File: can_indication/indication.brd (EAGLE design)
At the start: 63.5 x 38 mm, 51 parts, among them CON1 SM04B-GHS-TB, CON2 SM04B-GHS-TB, U1 STM32F103CB

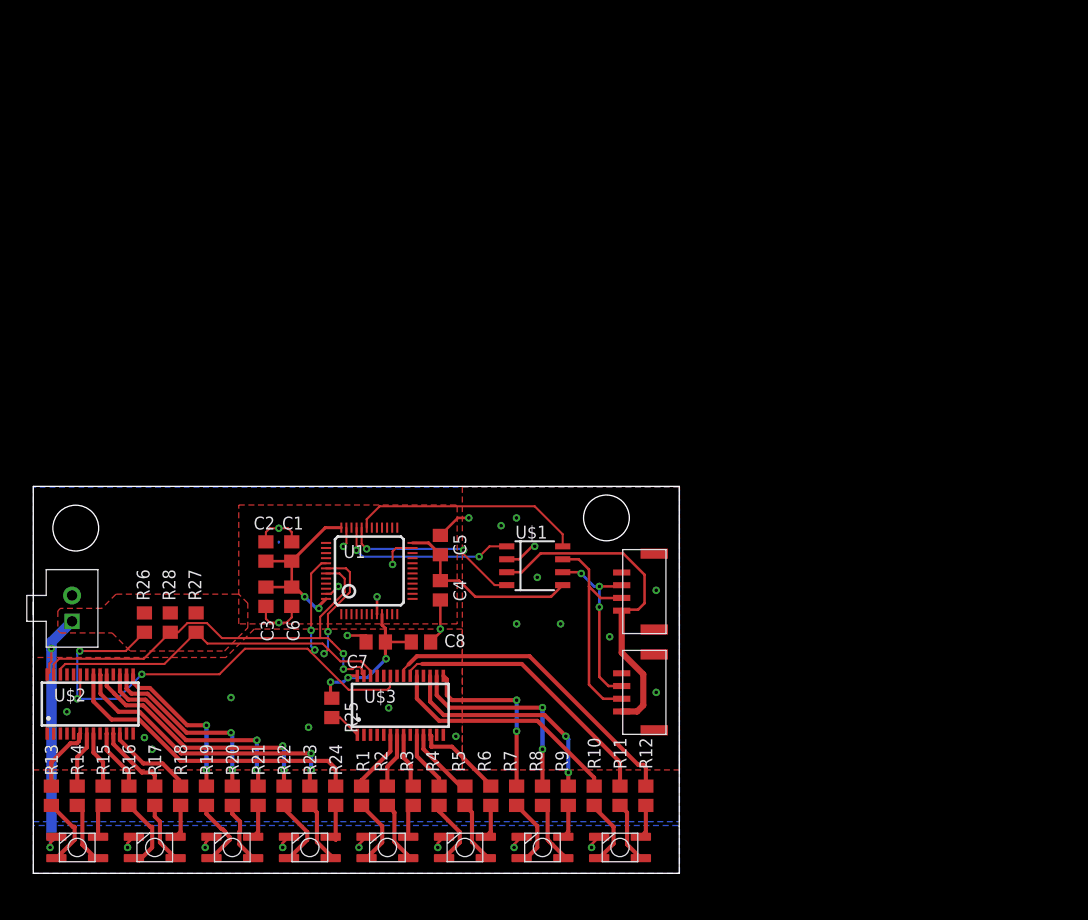
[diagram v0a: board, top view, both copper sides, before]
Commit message: Changed the indication board so it uses higher power LED's now
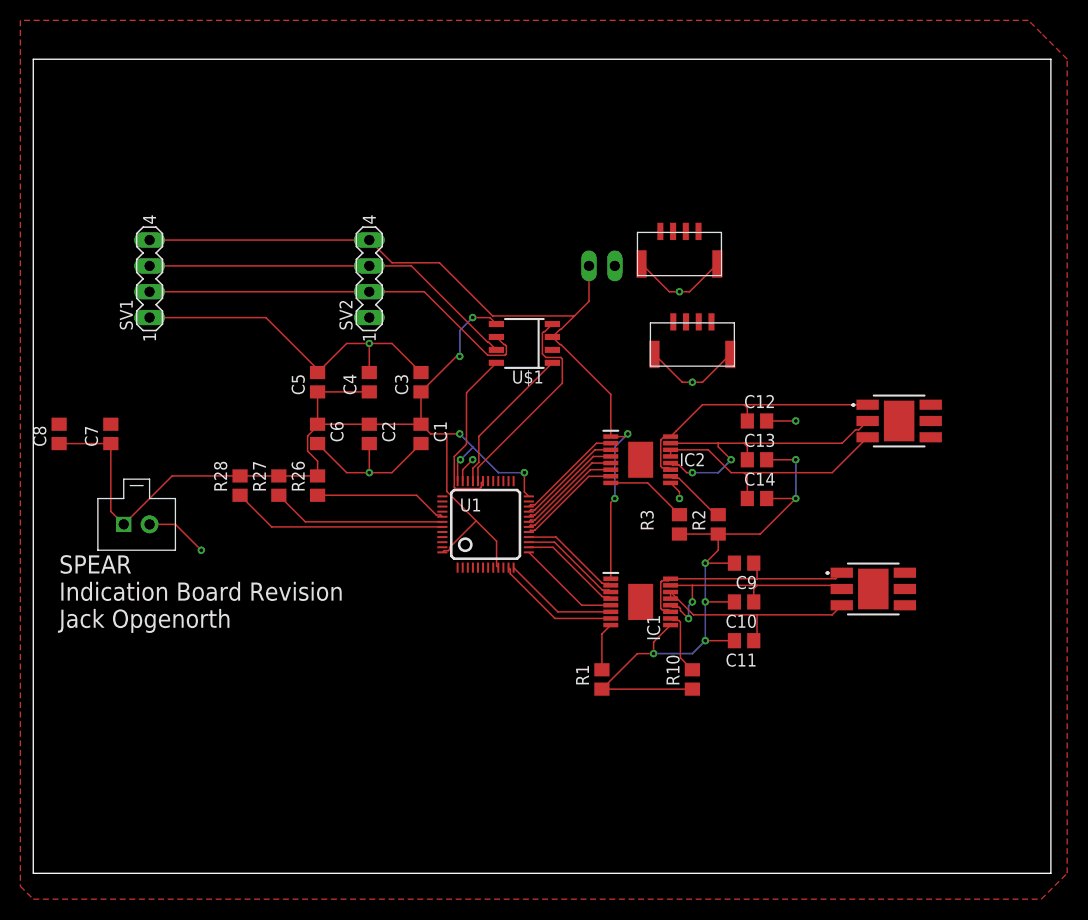
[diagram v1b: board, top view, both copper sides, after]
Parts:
- removed D1, D2, D3, D4, D5, D6, D7, D8: CLV1L-FKB-CHMMQEHBB7673673, SPEAR:PLCC-4
- removed R11, R12, R14, R15, R17, R18, R20, R21, R23, R24, R5, R6, R8, R9: 10, resistor:R0805
- removed R13, R16, R19, R22, R4, R7: 66, resistor:R0805
- removed R25: 10K, resistor:R0805
- removed U$2, U$3: PCA9685PW, SPEAR:TSSOP28
- added C10, C11, C12, C13, C14, C9: (no value), rcl:C0805
- added IC1, IC2: TPS92630QPWPRQ1, TPS92630QPWPRQ1:SOP65P640X120-17N
- added JP1: (no value), pinhead:1X02
- added LED1, LED2: AAAF5051-05, AAAF5051-05:AAAF505105
- added SV1, SV2: (no value), con-lstb:MA04-1
- R1: value 66 -> 10K
- R10: value 66 -> 815
- R2: value 10 -> 815
- R3: value 10 -> 10K
- moved R2 42.1 mm to (67.3, 34.3), turned to 90 degrees
- moved C8 41.0 mm to (2.54, 43.2), turned to 90 degrees
- moved R3 37.4 mm to (63.5, 34.3), turned to 90 degrees
- moved CON1 36.1 mm to (64.8, 53.3), turned to 0 degrees
- moved CON2 34.9 mm to (63.5, 62.2), turned to 0 degrees
- moved C7 33.1 mm to (7.62, 43.2), turned to 90 degrees
- moved R1 26.2 mm to (55.9, 19.1), turned to 90 degrees
- moved C3 26.0 mm to (38.1, 48.3), turned to 90 degrees
- moved U$1 21.9 mm to (48.3, 52.1), turned to 90 degrees
- moved R26 21.7 mm to (27.9, 38.1)
- moved C4 21.6 mm to (33.0, 48.3), turned to 90 degrees
- moved C5 20.0 mm to (27.9, 48.3)
- moved C1 17.2 mm to (38.1, 43.2), turned to 270 degrees
- moved C6 16.2 mm to (27.9, 43.2)
- moved R27 15.7 mm to (24.1, 38.1)
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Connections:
- removed net LEDA0: R13.1, U$2.6
- removed net LEDA1: R14.1, U$2.7
- removed net LEDA10: R21.1, U$2.17
- removed net LEDA11: U$2.18
- removed net LEDA12: R22.1, U$2.19
- removed net LEDA13: R23.1, U$2.20
- removed net LEDA14: R24.1, U$2.21
- removed net LEDA15: U$2.22
- removed net LEDA2: R15.1, U$2.8
- removed net LEDA3: U$2.9
- removed net LEDA4: R16.1, U$2.10
- removed net LEDA5: R17.1, U$2.11
- removed net LEDA6: R18.1, U$2.12
- removed net LEDA7: U$2.13
- removed net LEDA8: R19.1, U$2.15
- removed net LEDA9: R20.1, U$2.16
- removed net LEDB0: R1.1, U$3.6
- removed net LEDB1: R2.1, U$3.7
- removed net LEDB10: R9.1, U$3.17
- removed net LEDB11: U$3.18
- removed net LEDB12: R10.1, U$3.19
- removed net LEDB13: R11.1, U$3.20
- removed net LEDB14: R12.1, U$3.21
- removed net LEDB15: U$3.22
- removed net LEDB2: R3.1, U$3.8
- removed net LEDB3: U$3.9
- removed net LEDB4: R4.1, U$3.10
- removed net LEDB5: R5.1, U$3.11
- removed net LEDB6: R6.1, U$3.12
- removed net LEDB7: U$3.13
- removed net LEDB8: R7.1, U$3.15
- removed net LEDB9: R8.1, U$3.16
- removed net N$10: D8.P$2, R10.2
- removed net N$11: D8.P$3, R11.2
- removed net N$13: D1.P$2, R13.2
- removed net N$15: D1.P$4, R15.2
- removed net N$16: D2.P$2, R16.2
- removed net N$17: D2.P$3, R17.2
- removed net N$18: D2.P$4, R18.2
- removed net N$19: D3.P$2, R19.2
- removed net N$20: D3.P$3, R20.2
- removed net N$21: D3.P$4, R21.2
- removed net N$22: D4.P$2, R22.2
- removed net N$23: D4.P$3, R23.2
- removed net N$24: D4.P$4, R24.2
- removed net N$27: R25.2, U$3.1
- removed net N$4: D6.P$2, R4.2
- removed net N$5: D6.P$3, R5.2
- removed net N$6: D6.P$4, R6.2
- removed net N$7: D7.P$2, R7.2
- removed net N$8: D7.P$3, R8.2
- removed net N$9: D7.P$4, R9.2
- new net L1OUT1: C9.1, IC1.11, IC1.16, LED1.1
- new net L1OUT2: C10.1, IC1.12, IC1.15, LED1.2
- new net L1OUT3: C11.1, IC1.13, IC1.14, LED1.3
- new net L2OUT1: C12.1, IC2.11, IC2.16, LED2.1
- new net L2OUT2: C13.1, IC2.12, IC2.15, LED2.2
- new net L2OUT3: C14.1, IC2.13, IC2.14, LED2.3
- new net PA1: IC1.7, U1.11
- new net PA2: IC1.6, U1.12
- new net PA3: IC1.5, U1.13
- new net PA4: IC1.4, U1.14
- new net PA5: IC1.3, U1.15
- new net PA6: IC1.2, U1.16
- new net PA7: IC2.7, U1.17
- new net PB0: IC2.6, U1.18
- new net PB1: IC2.5, U1.19
- new net PB10: IC2.3, U1.21
- new net PB11: IC2.2, U1.22
- new net PB2: IC2.4, U1.20
- new net PB8: U1.45
- net +3V3: no longer D1.P$1, D2.P$1, D3.P$1, D4.P$1, D5.P$1, D6.P$1, D7.P$1, D8.P$1, R25.1, U$2.28, U$3.28
- net +5V: now also IC1.1, IC2.1, JP1.1, SV1.4, SV2.4; no longer CON1.P$1, CON2.P$1
- net CANH: now also SV1.3, SV2.3; no longer CON1.P$2, CON2.P$2
- net CANL: now also SV1.2, SV2.2; no longer CON1.P$3, CON2.P$3
- net GND: now also C10.2, C11.2, C12.2, C13.2, C14.2, C9.2, IC1.9, IC2.9, JP1.2, R1.1, R10.1, R2.1, R3.1, SV1.1, SV2.1; no longer CON1.P$4, CON2.P$4, U$2.1, U$2.14, U$2.2, U$2.24, U$2.3, U$2.4, U$2.5, U$3.14, U$3.2, U$3.24, U$3.3, U$3.4, U$3.5
- net I2C_SCL: no longer U$2.26, U$3.26
- net I2C_SDA: no longer U$2.27, U$3.27
- net LED_!OE: no longer U$2.23, U$3.23
- net N$1: now also IC1.10, R10.2; no longer D5.P$2, R1.2
- net N$12: now also IC1.8, R1.2; no longer D8.P$4, R12.2
- net N$14: now also U1.46; no longer D1.P$3, R14.2
- net N$2: now also IC2.8, R3.2; no longer D5.P$3, R2.2
- net N$3: now also IC2.10, R2.2; no longer D5.P$4, R3.2
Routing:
- net GND: track 32.4 -> 148.9 mm, vias 25 -> 14
- net +5V: track 33.3 -> 82.3 mm, vias 0 -> 2
- net LED_!OE: track 60.1 -> 13.1 mm, vias 5 -> 0
- net LEDB14: track 31.3 -> 0.00 mm
- net L2OUT2: track 0.00 -> 31.0 mm, vias 0 -> 2
- net LEDA14: track 30.9 -> 0.00 mm
- net I2C_SCL: track 46.7 -> 17.2 mm, vias 2 -> 0
- net LEDA13: track 28.3 -> 0.00 mm, vias 2 -> 0
- net LEDB13: track 27.7 -> 0.00 mm
- net L2OUT1: track 0.00 -> 27.2 mm
- net L2OUT3: track 0.00 -> 25.1 mm
- net LEDA12: track 25.0 -> 0.00 mm, vias 2 -> 0
- net L1OUT2: track 0.00 -> 24.6 mm, vias 0 -> 2
- net I2C_SDA: track 45.5 -> 21.2 mm, vias 2 -> 0
- net +3V3: track 89.0 -> 112.8 mm, vias 14 -> 5
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- removed copper zone on layer 1, net +3V3
- removed copper zone on layer 16, net +3V3
- removed copper zone on layer 16, net GND
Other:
- board size 63.5 x 38 mm -> 100 x 80 mm
- board text added: "SPEAR Indication Board Revision Jack Opgenorth"
